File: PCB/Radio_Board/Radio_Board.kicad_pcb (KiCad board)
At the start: 2 copper layers, 90 x 90 mm, 2 parts, among them J1 Conn_02x08_Counter_Clockwise, J2 SE2-30

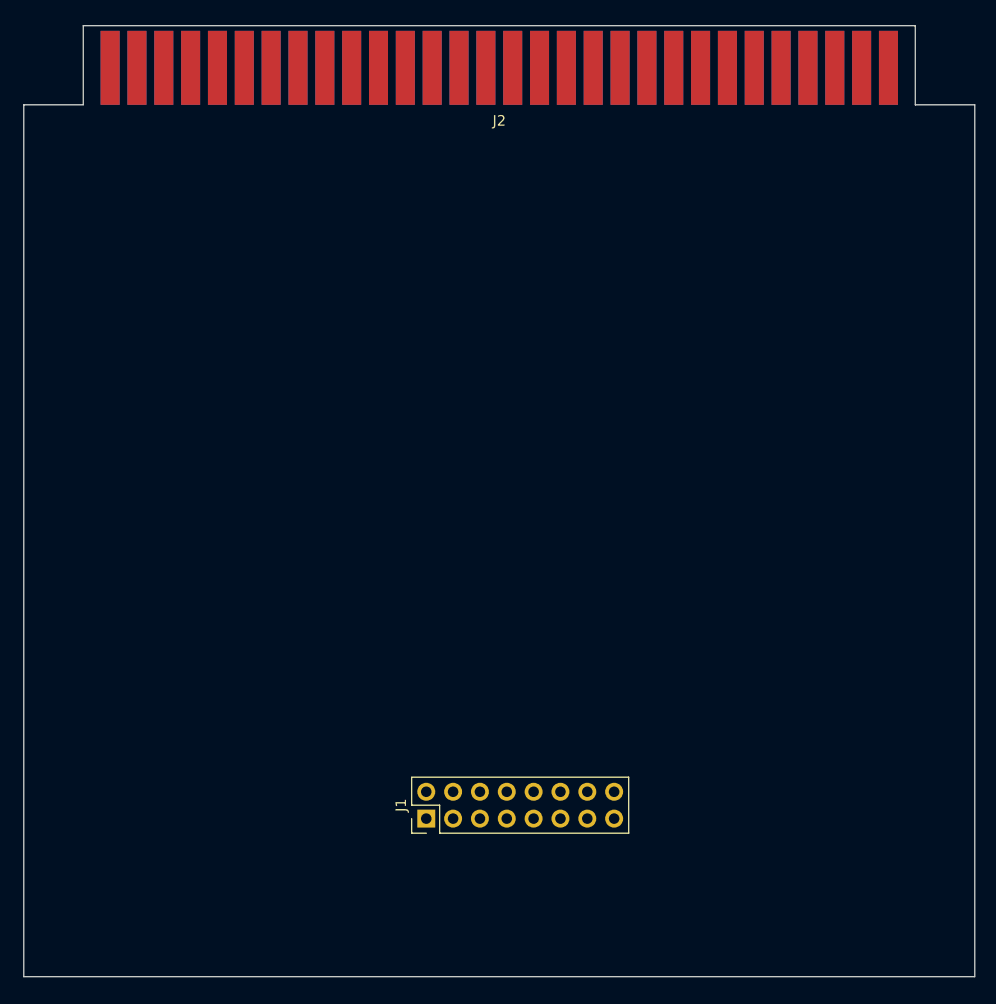
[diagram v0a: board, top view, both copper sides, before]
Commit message: Wired Layout
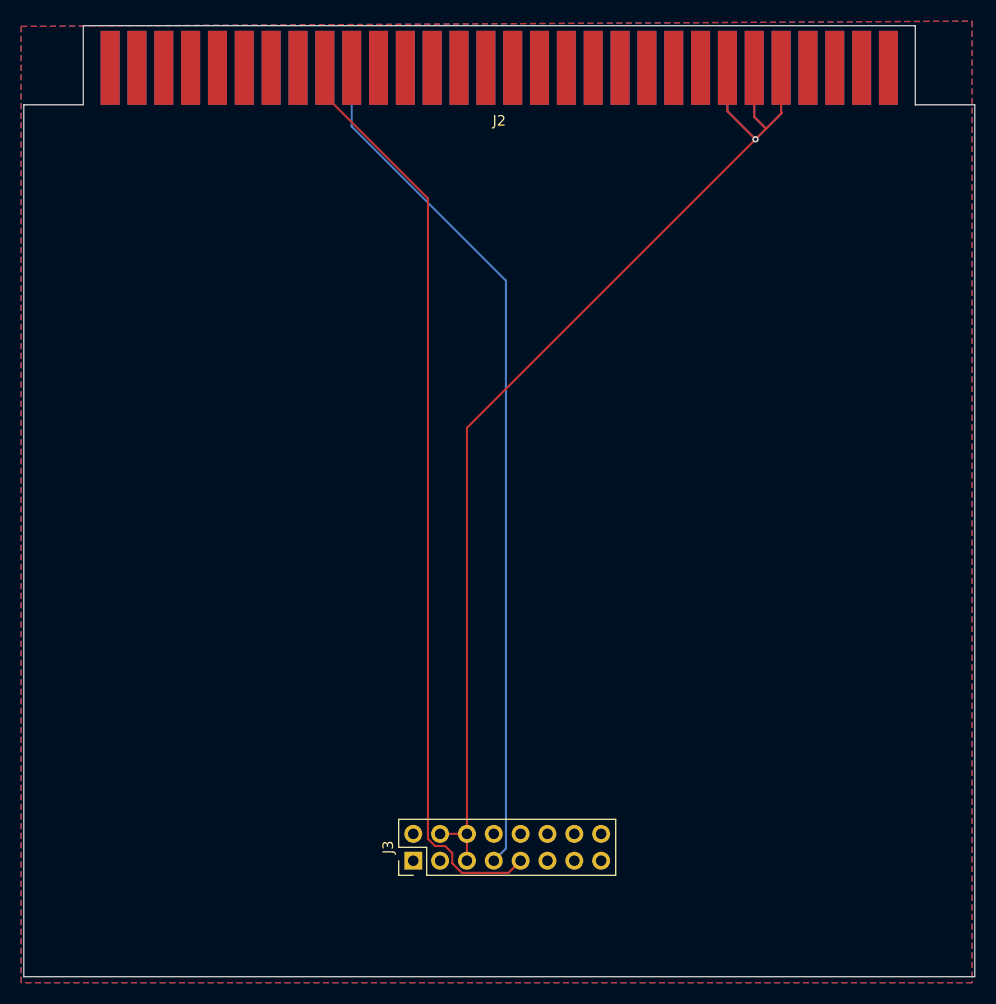
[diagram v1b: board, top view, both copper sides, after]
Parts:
- removed J1: Conn_02x08_Counter_Clockwise, Connector_PinHeader_2.54mm:PinHeader_2x08_P2.54mm_Vertical
- added J3: Conn_02x08_Odd_Even, Connector_PinHeader_2.54mm:PinHeader_2x08_P2.54mm_Vertical, F.Cu at (140.6, 131.3)
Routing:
- net +5V: track 0.00 -> 125.9 mm, vias 0 -> 1
- net /Tx: track 0.00 -> 88.2 mm
- net /Rx: track 0.00 -> 81.6 mm
- added copper zone on B.Cu, net GND
- added copper zone on F.Cu, net GND
